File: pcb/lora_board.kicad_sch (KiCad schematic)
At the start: 32 parts, among them J1 USB_C_Receptacle_USB2.0_16P, J2 Conn_01x02_Shielded, J3 Conn_01x05, J4 Qi Charger, Q1 AO3400A, SW1 SW_Push, SW2 SW_SPDT, U1 E73-2G4M08S1C, U2 AP2112K-3.3, U3 E22-900MM22S, U4 MCP73831-2-OT

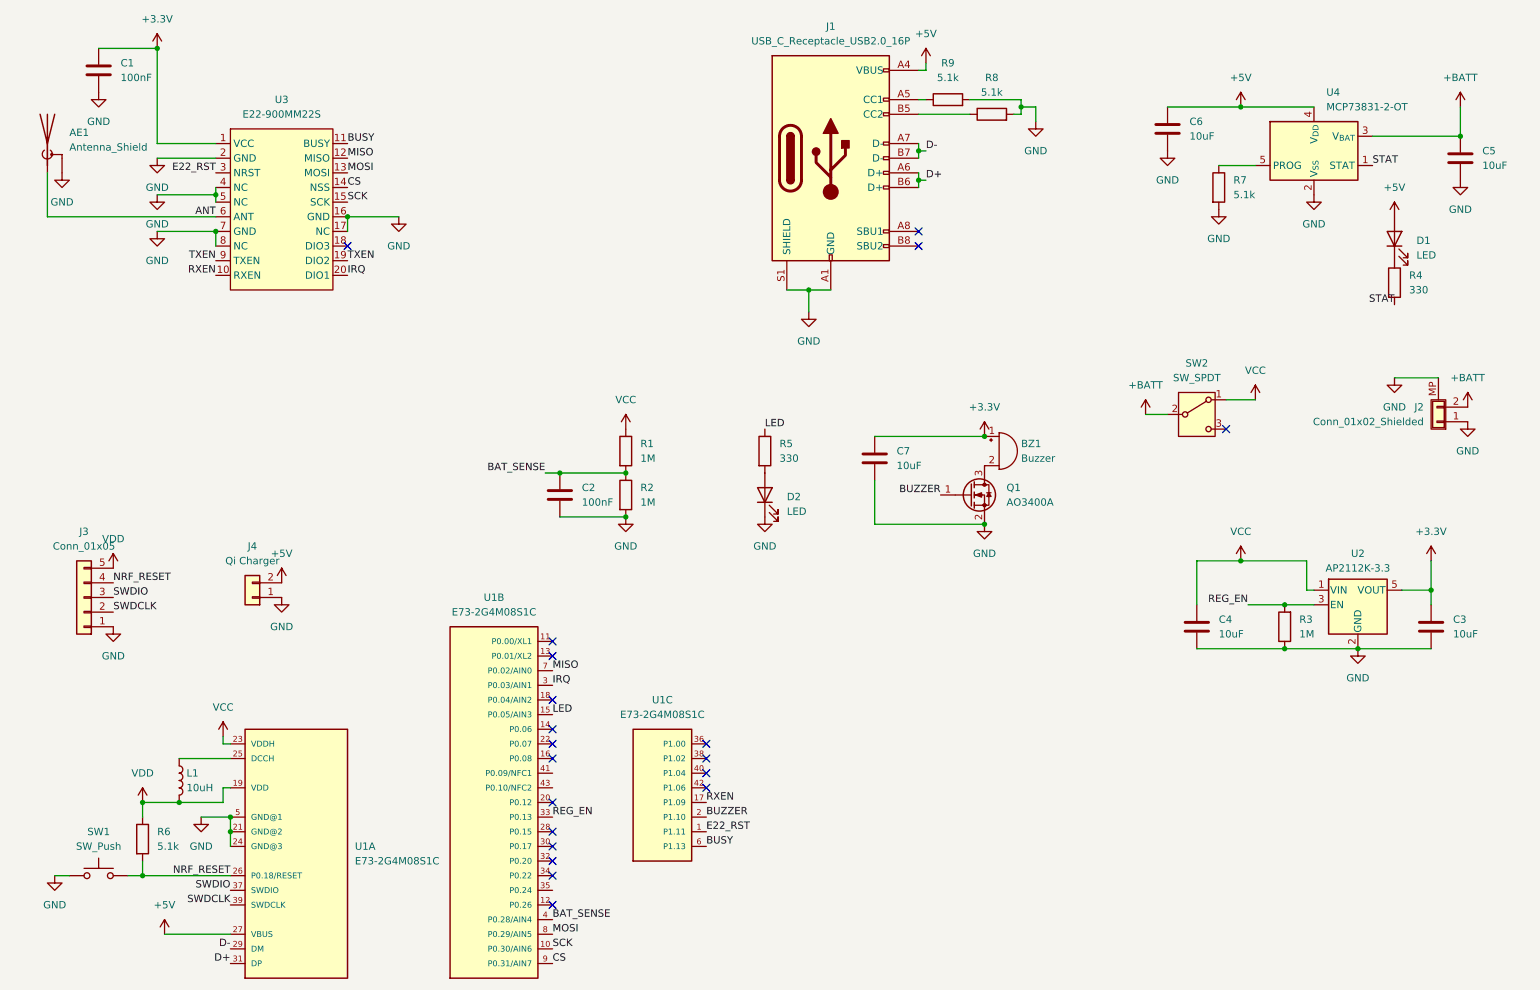
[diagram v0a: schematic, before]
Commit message: ordered v2
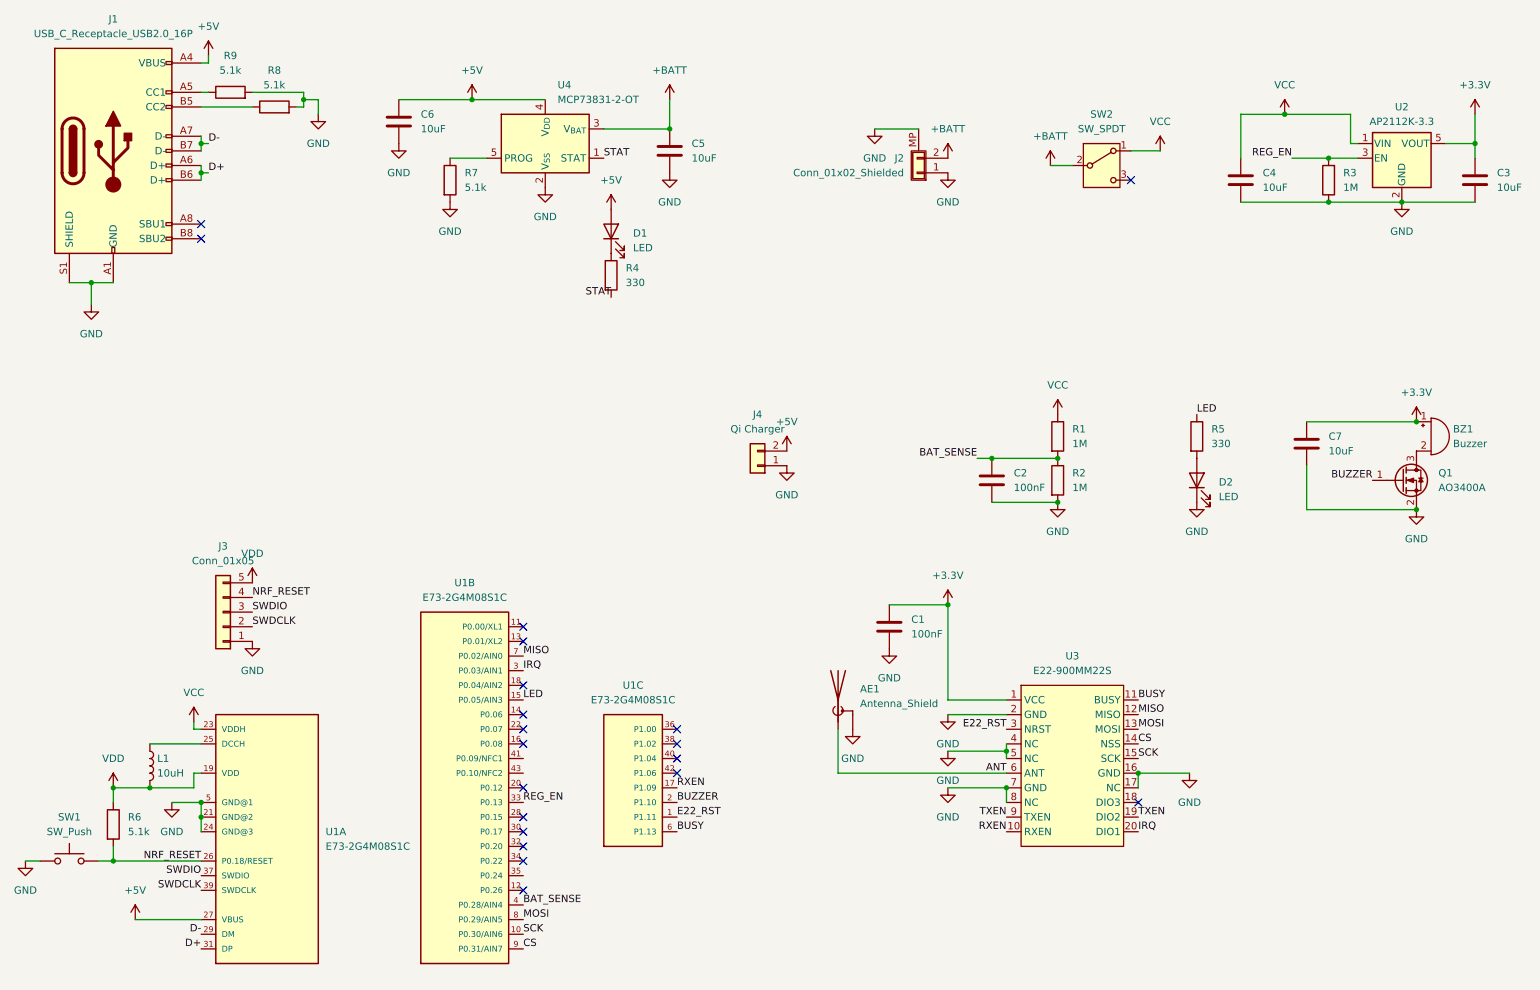
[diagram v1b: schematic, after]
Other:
- moved on the sheet: AE1, BZ1, C1, C2, C3, C4, C5, C6, C7, D1, D2, J1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
